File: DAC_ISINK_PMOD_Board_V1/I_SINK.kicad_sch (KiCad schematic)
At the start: 11 parts, among them Q1 MMBTA44, U3 OPA333xxDCK

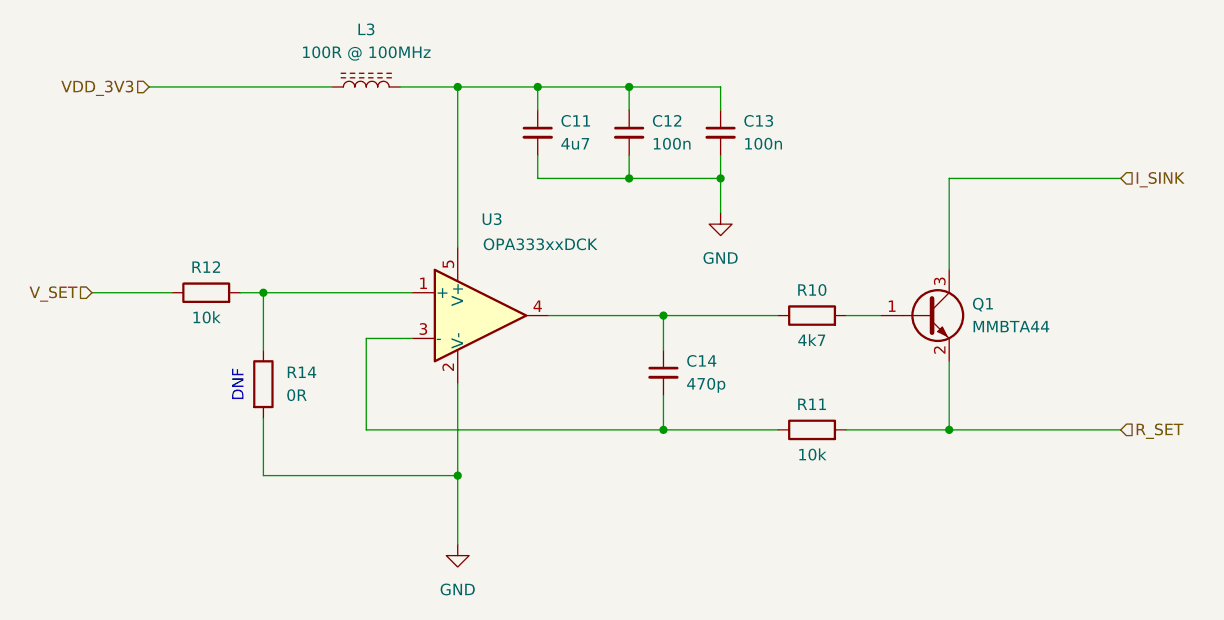
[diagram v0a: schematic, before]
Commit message: Manufacturing Data Generated.
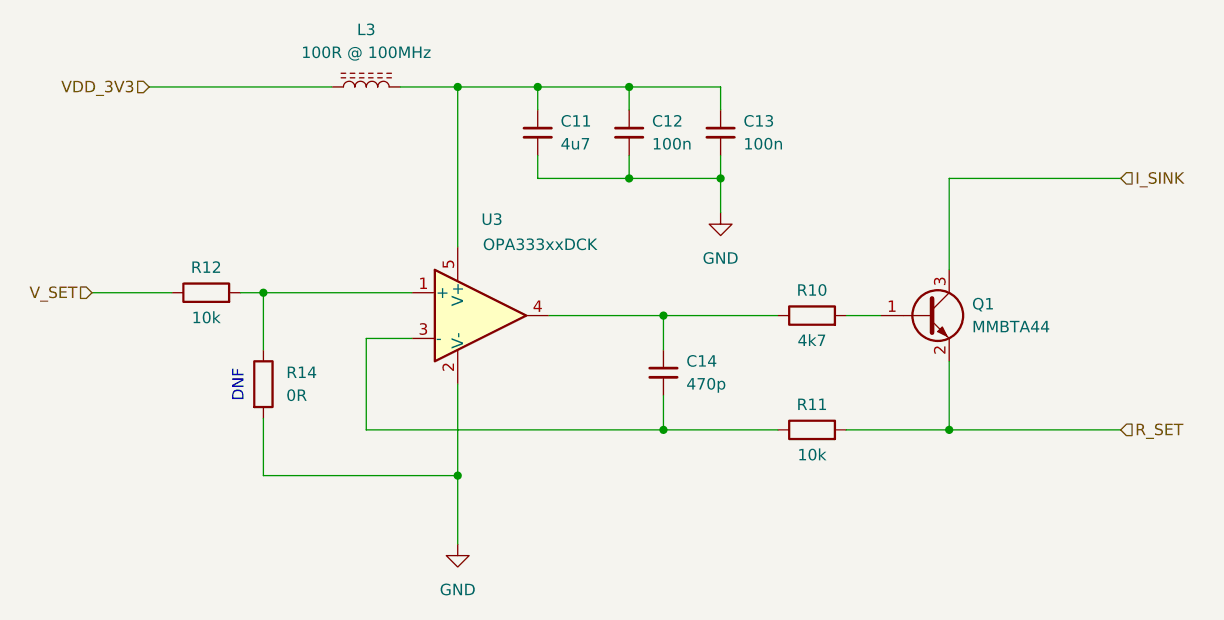
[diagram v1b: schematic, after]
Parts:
- C11, C12, C13, C14: footprint (none) -> Capacitor_SMD:C_0603_1608Metric
- L3: footprint (none) -> Inductor_SMD:L_0603_1608Metric
- R10, R11, R12: footprint (none) -> Resistor_SMD:R_0603_1608Metric
- R14: footprint Resistor_SMD:R_0402_1005Metric -> Resistor_SMD:R_0603_1608Metric
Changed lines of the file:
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@@
 			)
 		)
-		(property "Footprint" "Resistor_SMD:R_0402_1005Metric"
+		(property "Footprint" "Resistor_SMD:R_0603_1608Metric"
 			(at 99.822 96.52 90)
 			(hide yes)
@@
 			)
 		)
-		(property "Footprint" ""
+		(property "Footprint" "Inductor_SMD:L_0603_1608Metric"
 			(at 113.03 63.5 0)
 			(hide yes)
@@
 			)
 		)
-		(property "Footprint" ""
+		(property "Footprint" "Resistor_SMD:R_0603_1608Metric"
 			(at 162.56 90.678 90)
 			(hide yes)
@@
 			)
 		)
-		(property "Footprint" ""
+		(property "Footprint" "Capacitor_SMD:C_0603_1608Metric"
 			(at 142.24 68.58 0)
 			(hide yes)
@@
 			)
 		)
-		(property "Footprint" ""
+		(property "Footprint" "Resistor_SMD:R_0603_1608Metric"
 			(at 95.25 88.138 90)
 			(hide yes)
@@
 			)
 		)
-		(property "Footprint" ""
+		(property "Footprint" "Capacitor_SMD:C_0603_1608Metric"
 			(at 146.05 95.25 0)
 			(hide yes)
@@
 			)
 		)
-		(property "Footprint" ""
+		(property "Footprint" "Capacitor_SMD:C_0603_1608Metric"
 			(at 132.08 68.58 0)
 			(hide yes)
@@
 			)
 		)
-		(property "Footprint" ""
+		(property "Footprint" "Resistor_SMD:R_0603_1608Metric"
 			(at 162.56 103.378 90)
 			(hide yes)
@@
 			)
 		)
-		(property "Footprint" ""
+		(property "Footprint" "Capacitor_SMD:C_0603_1608Metric"
 			(at 152.4 68.58 0)
 			(hide yes)
